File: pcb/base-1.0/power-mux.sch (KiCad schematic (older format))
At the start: 26 parts, among them Q201 Q_PMOS_DGS, Q202 Q_PMOS_DGS, Q203 Q_PMOS_DGS, Q204 Q_PMOS_DGS, Q205 Q_PMOS_DGS, Q206 Q_PMOS_DGS, U201 LTC4417

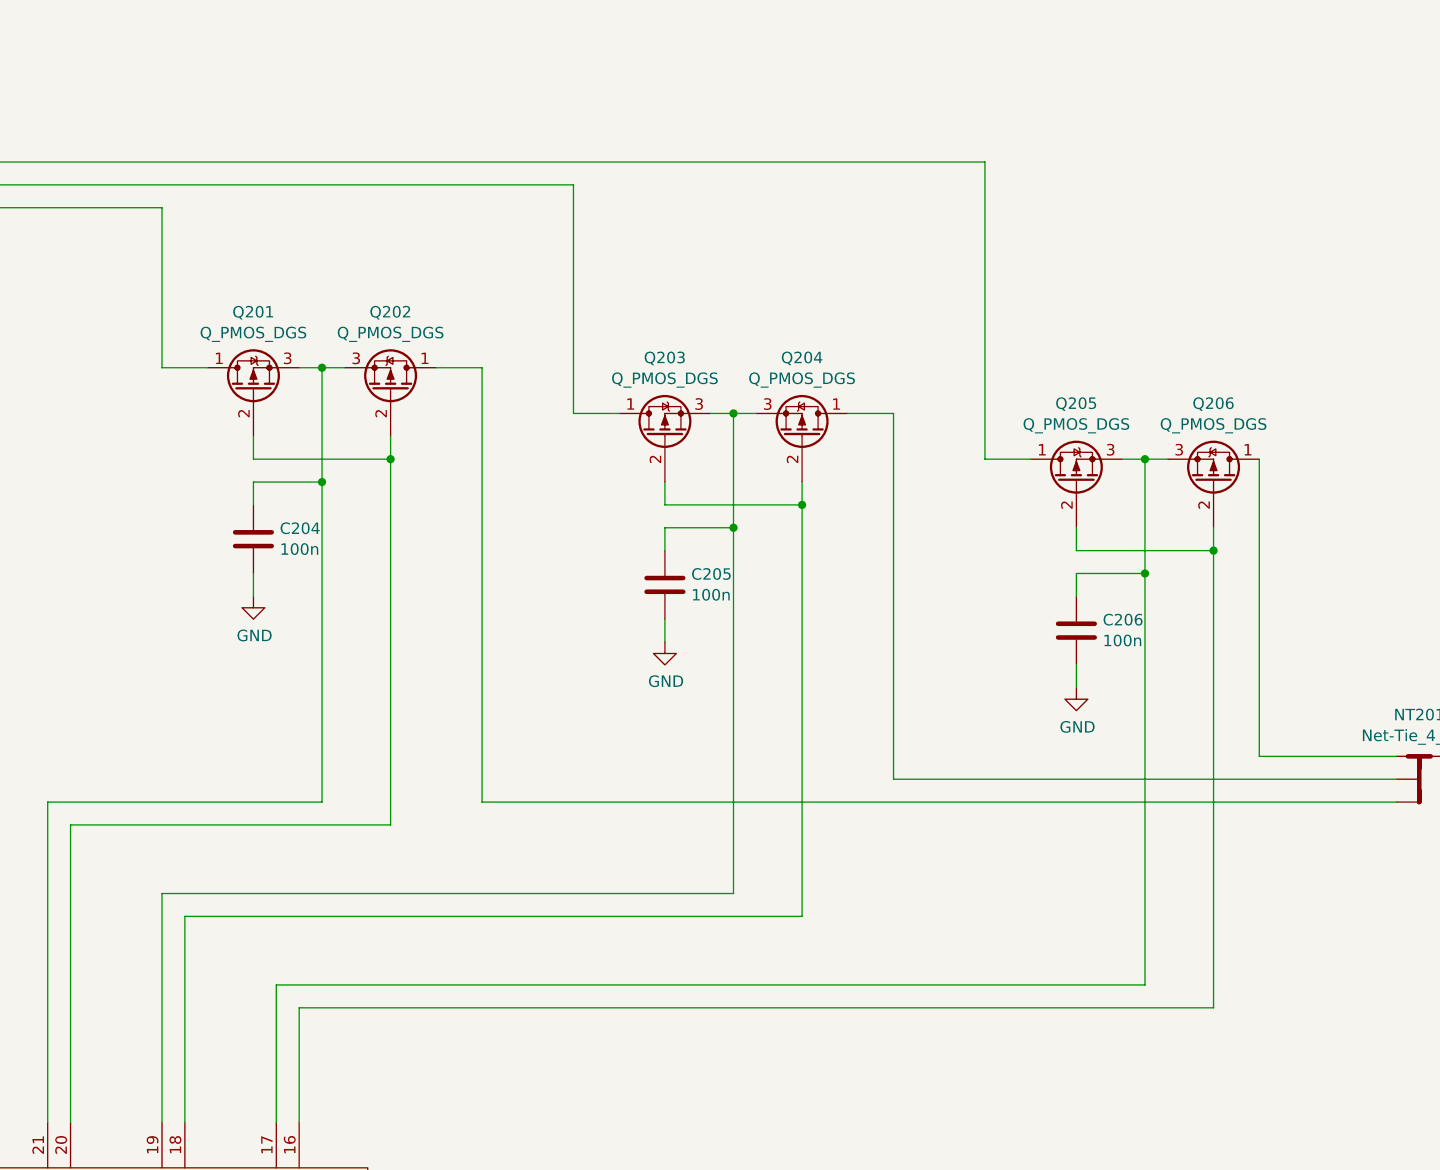
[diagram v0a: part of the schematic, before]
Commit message: wip
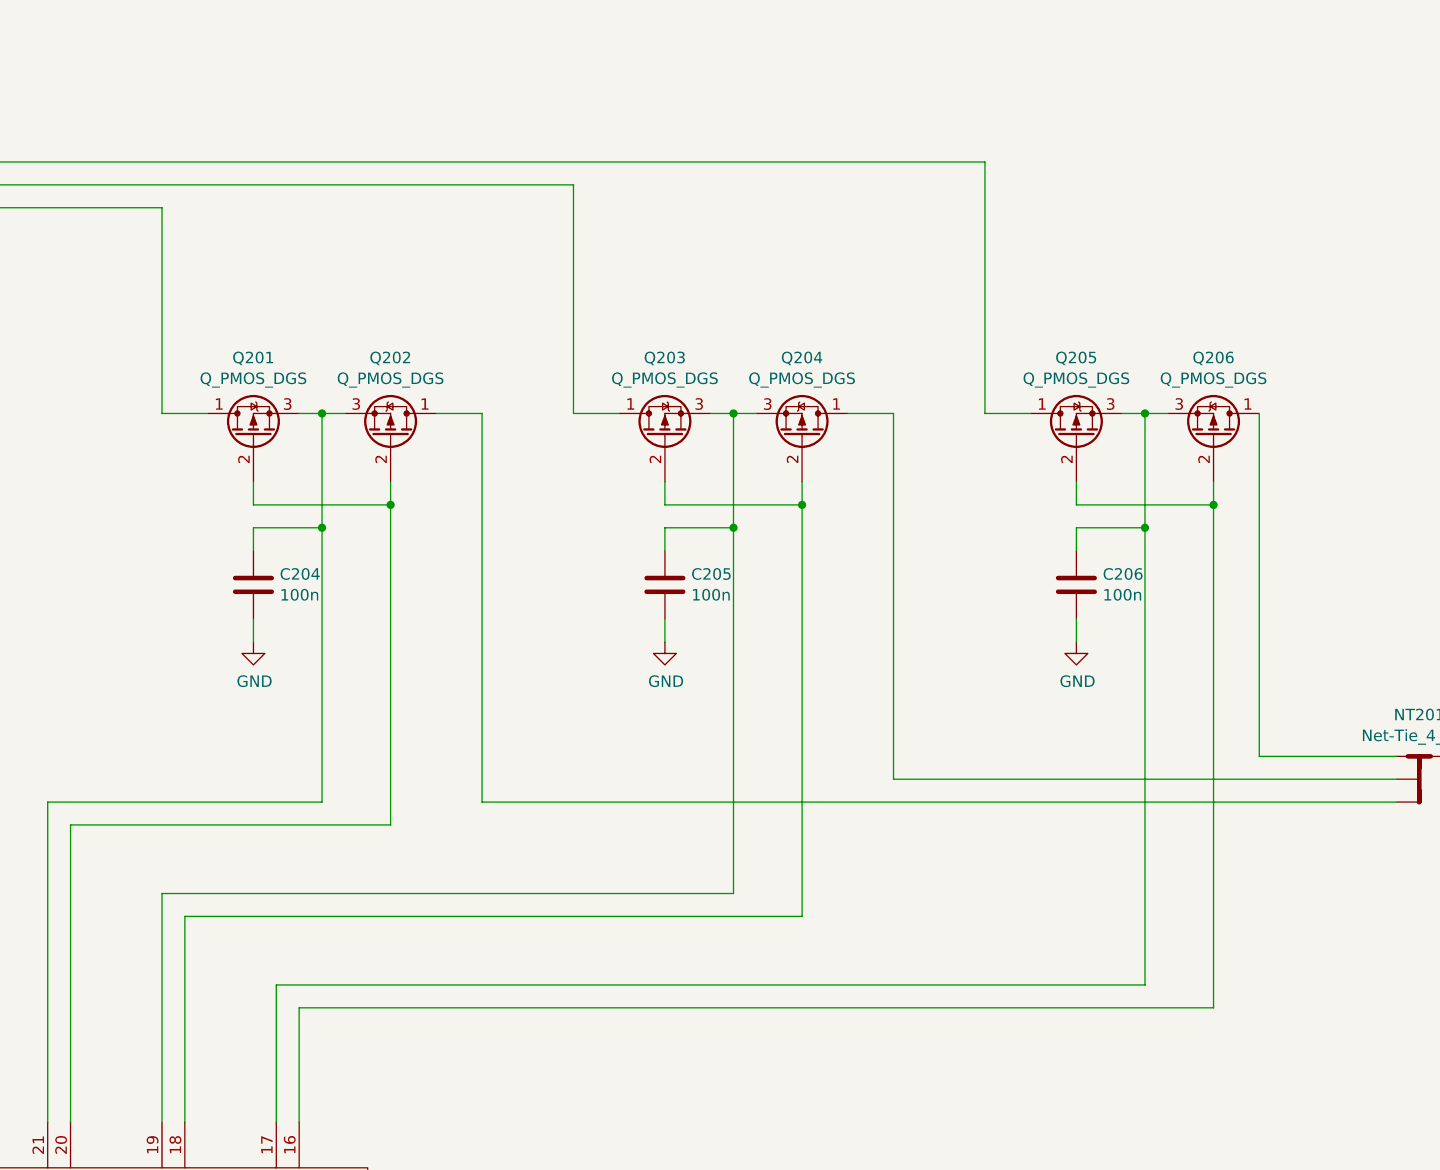
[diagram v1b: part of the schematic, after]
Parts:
- Q201, Q202, Q203, Q204, Q205, Q206: mpn (none) -> IRF7324TRPBF
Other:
- moved on the sheet: C204, C206, Q201, Q202, Q205, Q206
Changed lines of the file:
@@
 L Device:Q_PMOS_DGS Q201
 U 1 1 5CF241D9
-P 4900 1800
-F 0 "Q201" V 5243 1800 50  0000 C CNN
-F 1 "Q_PMOS_DGS" V 5152 1800 50  0000 C CNN
-F 2 "" H 5100 1900 50  0001 C CNN
-F 3 "~" H 4900 1800 50  0001 C CNN
-	1    4900 1800
+P 4900 2000
+F 0 "Q201" V 5243 2000 50  0000 C CNN
+F 1 "Q_PMOS_DGS" V 5152 2000 50  0000 C CNN
+F 2 "" H 5100 2100 50  0001 C CNN
+F 3 "~" H 4900 2000 50  0001 C CNN
+F 4 "IRF7324TRPBF" H 4900 2000 50  0001 C CNN "mpn"
+	1    4900 2000
 	0    -1   -1   0
 $EndComp
 Wire Wire Line
-	5100 1700 5200 1700
-Wire Wire Line
-	5200 1700 5200 2200
-Connection ~ 5200 1700
-Wire Wire Line
-	5200 1700 5300 1700
-Wire Wire Line
-	4900 2000 4900 2100
-Wire Wire Line
-	4900 2100 5500 2100
-Wire Wire Line
-	5500 2100 5500 2000
-Connection ~ 5500 2100
-Wire Wire Line
-	4900 2200 5200 2200
-Connection ~ 5200 2200
+	5100 1900 5200 1900
+Wire Wire Line
+	5200 1900 5200 2400
+Connection ~ 5200 1900
+Wire Wire Line
+	5200 1900 5300 1900
+Wire Wire Line
+	4900 2200 4900 2300
+Wire Wire Line
+	4900 2300 5500 2300
+Wire Wire Line
+	5500 2300 5500 2200
+Connection ~ 5500 2300
+Wire Wire Line
+	4900 2400 5200 2400
+Connection ~ 5200 2400
 $Comp
 L Device:C C204
 U 1 1 5CF2798D
-P 4900 2450
-F 0 "C204" H 5015 2496 50  0000 L CNN
-F 1 "100n" H 5015 2405 50  0000 L CNN
-F 2 "Capacitor_SMD:C_0402_1005Metric" H 4938 2300 50  0001 C CNN
-F 3 "~" H 4900 2450 50  0001 C CNN
-	1    4900 2450
-	1    0    0    -1
-$EndComp
-Wire Wire Line
-	4900 2200 4900 2300
+P 4900 2650
+F 0 "C204" H 5015 2696 50  0000 L CNN
+F 1 "100n" H 5015 2605 50  0000 L CNN
+F 2 "Capacitor_SMD:C_0402_1005Metric" H 4938 2500 50  0001 C CNN
+F 3 "~" H 4900 2650 50  0001 C CNN
+	1    4900 2650
+	1    0    0    -1
+$EndComp
+Wire Wire Line
+	4900 2400 4900 2500
 $Comp
 L power:GND #PWR0112
 U 1 1 5CF2B26C
-P 4900 2700
-F 0 "#PWR0112" H 4900 2450 50  0001 C CNN
-F 1 "GND" H 4905 2527 50  0000 C CNN
-F 2 "" H 4900 2700 50  0001 C CNN
-F 3 "" H 4900 2700 50  0001 C CNN
-	1    4900 2700
-	1    0    0    -1
-$EndComp
-Wire Wire Line
-	4900 2700 4900 2600
+P 4900 2900
+F 0 "#PWR0112" H 4900 2650 50  0001 C CNN
+F 1 "GND" H 4905 2727 50  0000 C CNN
+F 2 "" H 4900 2900 50  0001 C CNN
+F 3 "" H 4900 2900 50  0001 C CNN
+	1    4900 2900
+	1    0    0    -1
+$EndComp
+Wire Wire Line
+	4900 2900 4900 2800
 $Comp
 L Device:Q_PMOS_DGS Q203
@@
 F 2 "" H 6900 2100 50  0001 C CNN
 F 3 "~" H 6700 2000 50  0001 C CNN
+F 4 "IRF7324TRPBF" H 6700 2000 50  0001 C CNN "mpn"
 	1    6700 2000
 	0    -1   -1   0
@@
 F 2 "" H 7500 2100 50  0001 C CNN
 F 3 "~" H 7300 2000 50  0001 C CNN
+F 4 "IRF7324TRPBF" H 7300 2000 50  0001 C CNN "mpn"
 	1    7300 2000
 	0    1    -1   0
@@
 Wire Wire Line
 	6700 2900 6700 2800
-$Comp
-L Device:Q_PMOS_DGS Q205
-U 1 1 5CF45010
-P 8500 2200
-F 0 "Q205" V 8843 2200 50  0000 C CNN
-F 1 "Q_PMOS_DGS" V 8752 2200 50  0000 C CNN
-F 2 "" H 8700 2300 50  0001 C CNN
-F 3 "~" H 8500 2200 50  0001 C CNN
-	1    8500 2200
-	0    -1   -1   0
-$EndComp
-$Comp
-L Device:Q_PMOS_DGS Q206
-U 1 1 5CF45016
-P 9100 2200
-F 0 "Q206" V 9443 2200 50  0000 C CNN
-F 1 "Q_PMOS_DGS" V 9352 2200 50  0000 C CNN
-F 2 "" H 9300 2300 50  0001 C CNN
-F 3 "~" H 9100 2200 50  0001 C CNN
-	1    9100 2200
-	0    1    -1   0
-$EndComp
-Wire Wire Line
-	8700 2100 8800 2100
-Wire Wire Line
-	8800 2100 8800 2600
-Connection ~ 8800 2100
-Wire Wire Line
-	8800 2100 8900 2100
-Wire Wire Line
-	8500 2400 8500 2500
-Wire Wire Line
-	8500 2500 9100 2500
-Wire Wire Line
-	9100 2500 9100 2400
-Connection ~ 9100 2500
-Wire Wire Line
-	8500 2600 8800 2600
-Connection ~ 8800 2600
-$Comp
-L Device:C C206
-U 1 1 5CF45026
-P 8500 2850
-F 0 "C206" H 8615 2896 50  0000 L CNN
-F 1 "100n" H 8615 2805 50  0000 L CNN
-F 2 "Capacitor_SMD:C_0402_1005Metric" H 8538 2700 50  0001 C CNN
-F 3 "~" H 8500 2850 50  0001 C CNN
-	1    8500 2850
-	1    0    0    -1
-$EndComp
-Wire Wire Line
-	8500 2600 8500 2700
-$Comp
-L power:GND #PWR0114
-U 1 1 5CF4502D
-P 8500 3100
-F 0 "#PWR0114" H 8500 2850 50  0001 C CNN
-F 1 "GND" H 8505 2927 50  0000 C CNN
-F 2 "" H 8500 3100 50  0001 C CNN
-F 3 "" H 8500 3100 50  0001 C CNN
-	1    8500 3100
-	1    0    0    -1
-$EndComp
-Wire Wire Line
-	8500 3100 8500 3000
-Wire Wire Line
-	4500 1000 4500 1700
-Wire Wire Line
-	4500 1700 4700 1700
+Wire Wire Line
+	4500 1000 4500 1900
+Wire Wire Line
+	4500 1900 4700 1900
 Wire Wire Line
 	6300 900  6300 1900
@@
 	6300 1900 6500 1900
 Wire Wire Line
-	8100 2100 8300 2100
-Wire Wire Line
-	5700 1700 5900 1700
-Wire Wire Line
-	5900 1700 5900 3600
+	5700 1900 5900 1900
+Wire Wire Line
+	5900 1900 5900 3600
 Wire Wire Line
 	7500 1900 7700 1900
@@
 	7700 3500 9900 3500
 Wire Wire Line
-	9300 2100 9300 3400
-Wire Wire Line
 	9300 3400 9900 3400
 Wire Wire Line
-	9100 2500 9100 4500
-Wire Wire Line
-	8800 2600 8800 4400
-Wire Wire Line
 	4600 5000 4600 4100
 Wire Wire Line
@@
 	4100 5000 4100 3700
 Wire Wire Line
-	5500 2100 5500 3700
+	5500 2300 5500 3700
 Wire Wire Line
 	4000 5000 4000 3600
 Wire Wire Line
-	5200 2200 5200 3600
-Wire Wire Line
-	8100 800  8100 2100
+	5200 2400 5200 3600
 $Comp
 L Device:R R201
@@
 L Device:Q_PMOS_DGS Q202
 U 1 1 5CF24862
-P 5500 1800
-F 0 "Q202" V 5843 1800 50  0000 C CNN
-F 1 "Q_PMOS_DGS" V 5752 1800 50  0000 C CNN
-F 2 "" H 5700 1900 50  0001 C CNN
-F 3 "~" H 5500 1800 50  0001 C CNN
-	1    5500 1800
+P 5500 2000
+F 0 "Q202" V 5843 2000 50  0000 C CNN
+F 1 "Q_PMOS_DGS" V 5752 2000 50  0000 C CNN
+F 2 "" H 5700 2100 50  0001 C CNN
+F 3 "~" H 5500 2000 50  0001 C CNN
+F 4 "IRF7324TRPBF" H 5500 2000 50  0001 C CNN "mpn"
+	1    5500 2000
 	0    1    -1   0
 $EndComp
@@
 Wire Wire Line
 	4500 7300 4500 7200
+Wire Wire Line
+	8100 800  8100 1900
+Wire Wire Line
+	8800 2400 8800 4400
+Wire Wire Line
+	9100 2300 9100 4500
+Wire Wire Line
+	9300 1900 9300 3400
+Wire Wire Line
+	8100 1900 8300 1900
+Wire Wire Line
+	8500 2900 8500 2800
+$Comp
+L power:GND #PWR0114
+U 1 1 5CF4502D
+P 8500 2900
+F 0 "#PWR0114" H 8500 2650 50  0001 C CNN
+F 1 "GND" H 8505 2727 50  0000 C CNN
+F 2 "" H 8500 2900 50  0001 C CNN
+F 3 "" H 8500 2900 50  0001 C CNN
+	1    8500 2900
+	1    0    0    -1
+$EndComp
+Wire Wire Line
+	8500 2400 8500 2500
+$Comp
+L Device:C C206
+U 1 1 5CF45026
+P 8500 2650
+F 0 "C206" H 8615 2696 50  0000 L CNN
+F 1 "100n" H 8615 2605 50  0000 L CNN
+F 2 "Capacitor_SMD:C_0402_1005Metric" H 8538 2500 50  0001 C CNN
+F 3 "~" H 8500 2650 50  0001 C CNN
+	1    8500 2650
+	1    0    0    -1
+$EndComp
+Connection ~ 8800 2400
+Wire Wire Line
+	8500 2400 8800 2400
+Connection ~ 9100 2300
+Wire Wire Line
+	9100 2300 9100 2200
+Wire Wire Line
+	8500 2300 9100 2300
+Wire Wire Line
+	8500 2200 8500 2300
+Wire Wire Line
+	8800 1900 8900 1900
+Connection ~ 8800 1900
+Wire Wire Line
+	8800 1900 8800 2400
+Wire Wire Line
+	8700 1900 8800 1900
+$Comp
+L Device:Q_PMOS_DGS Q206
+U 1 1 5CF45016
+P 9100 2000
+F 0 "Q206" V 9443 2000 50  0000 C CNN
+F 1 "Q_PMOS_DGS" V 9352 2000 50  0000 C CNN
+F 2 "" H 9300 2100 50  0001 C CNN
+F 3 "~" H 9100 2000 50  0001 C CNN
+F 4 "IRF7324TRPBF" H 9100 2000 50  0001 C CNN "mpn"
+	1    9100 2000
+	0    1    -1   0
+$EndComp
+$Comp
+L Device:Q_PMOS_DGS Q205
+U 1 1 5CF45010
+P 8500 2000
+F 0 "Q205" V 8843 2000 50  0000 C CNN
+F 1 "Q_PMOS_DGS" V 8752 2000 50  0000 C CNN
+F 2 "" H 8700 2100 50  0001 C CNN
+F 3 "~" H 8500 2000 50  0001 C CNN
+F 4 "IRF7324TRPBF" H 8500 2000 50  0001 C CNN "mpn"
+	1    8500 2000
+	0    -1   -1   0
+$EndComp
 $EndSCHEMATC
